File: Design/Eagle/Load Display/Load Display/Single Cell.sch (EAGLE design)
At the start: 1 part

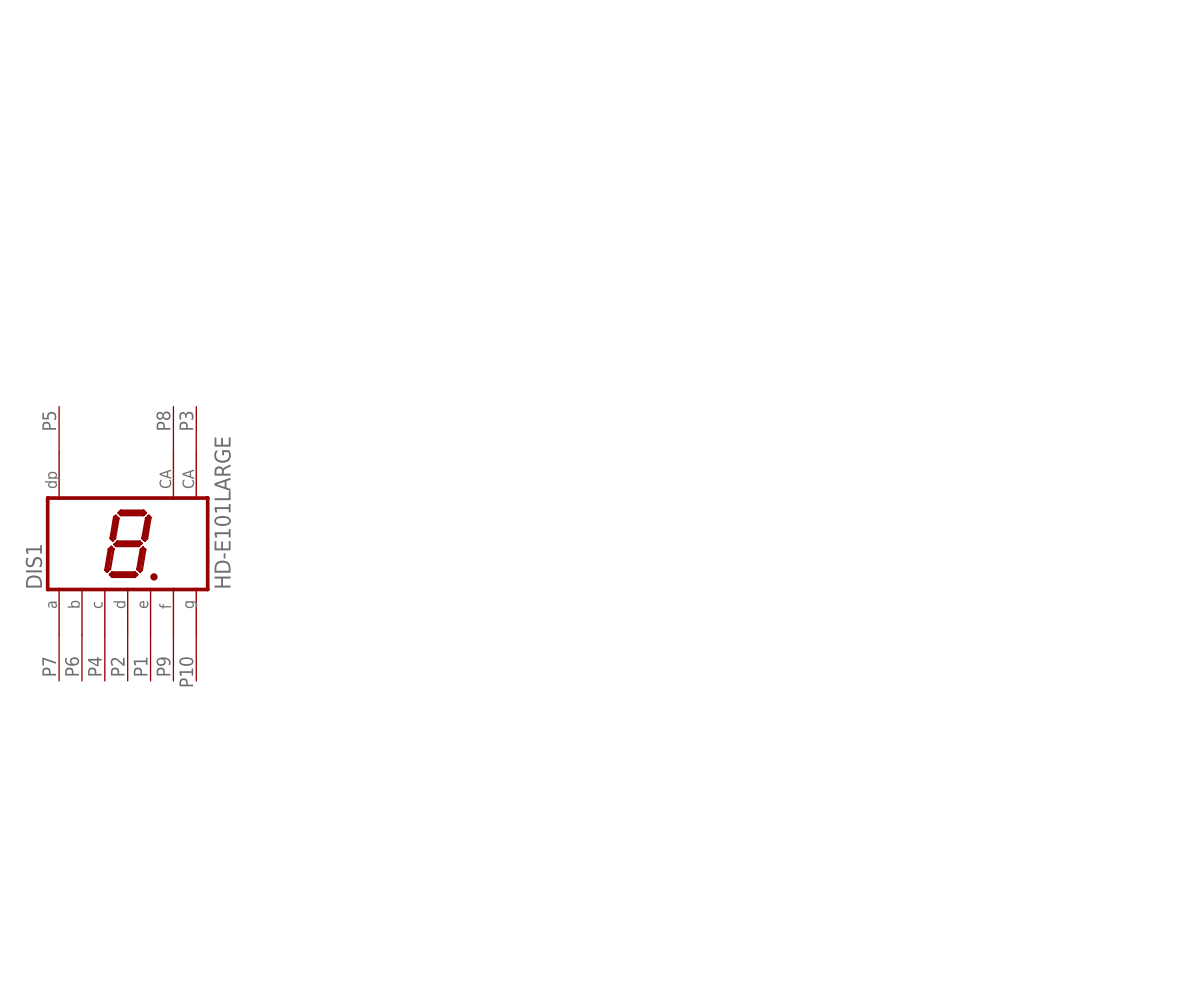
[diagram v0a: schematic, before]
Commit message: Added some eagle files
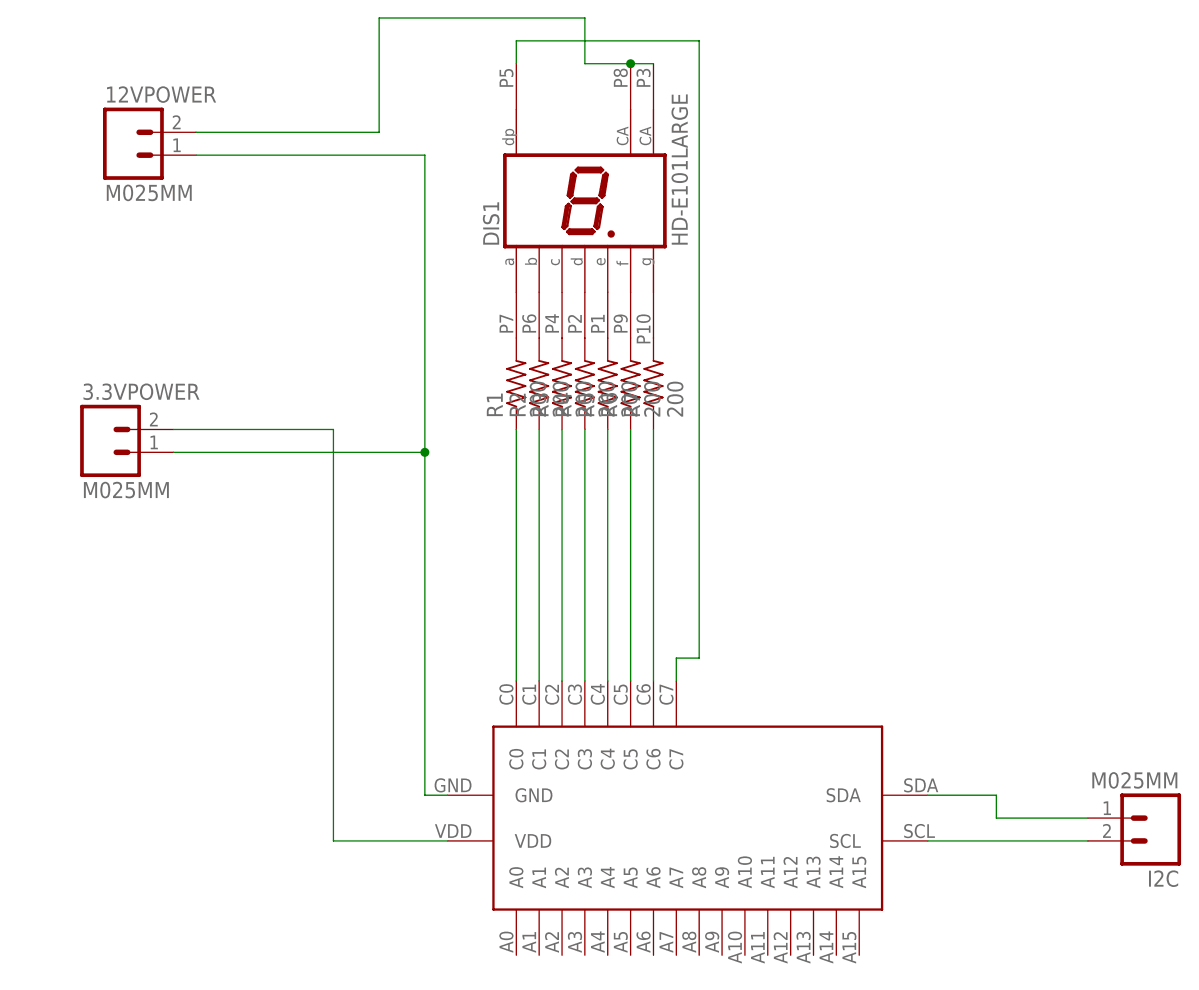
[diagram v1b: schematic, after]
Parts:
- added 12VPOWER, 3.3VPOWER, I2C: M025MM, Ben-SF-Con:M025MM
- added R1, R2, R3, R4, R5, R6, R7: 200, Ben-rcl:R-US_0207/10
- added U$3: HT16K33BRD, Parts:HT16K33BRD
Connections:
- new net N$1: DIS1.A, R1.2
- new net N$10: R3.1, U$3.C2
- new net N$11: R4.1, U$3.C3
- new net N$12: R5.1, U$3.C4
- new net N$13: R6.1, U$3.C5
- new net N$14: R7.1, U$3.C6
- new net N$15: I2C.1, U$3.SDA
- new net N$16: I2C.2, U$3.SCL
- new net N$17: 12VPOWER.1, 3.3VPOWER.1, U$3.GND
- new net N$18: DIS1.DP, U$3.C7
- new net N$19: 3.3VPOWER.2, U$3.VDD
- new net N$2: DIS1.B, R2.2
- new net N$20: 12VPOWER.2, DIS1.CA, DIS1.CA@1
- new net N$3: DIS1.C, R3.2
- new net N$4: DIS1.D, R4.2
- new net N$5: DIS1.E, R5.2
- new net N$6: DIS1.F, R6.2
- new net N$7: DIS1.G, R7.2
- new net N$8: R1.1, U$3.C0
- new net N$9: R2.1, U$3.C1
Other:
- moved on the sheet: DIS1
